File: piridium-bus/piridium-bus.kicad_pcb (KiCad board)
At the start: 2 copper layers, 90.2 x 95.9 mm, 53 parts, among them J1 EPS, J2 MODEM UART, J3 ANT, J4 PAYLOAD, Q1 2N7002, Q2 DMP3015LSSQ, U1 LM1117-3.3, U2 TPS54394RSAR, U3 MAX6369, U4 74LS126, U5 DS3232M

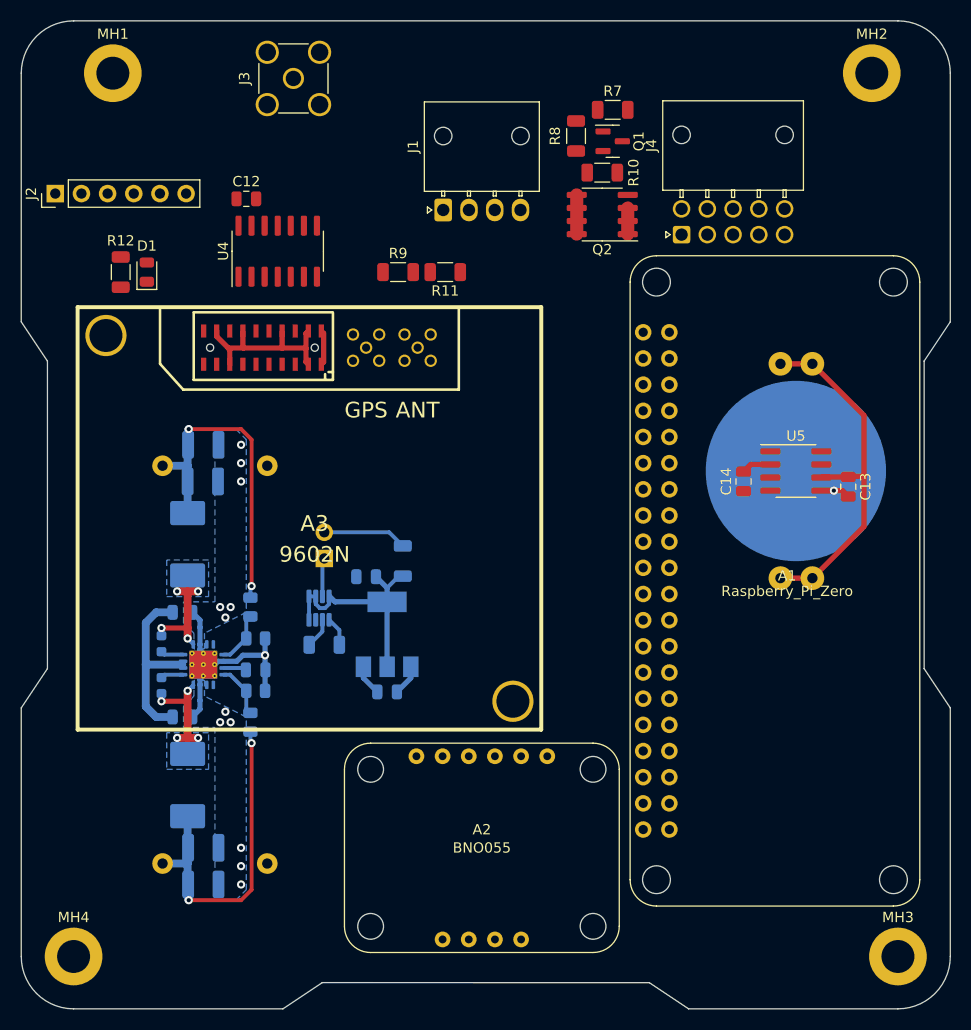
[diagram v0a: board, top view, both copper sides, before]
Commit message: update routing
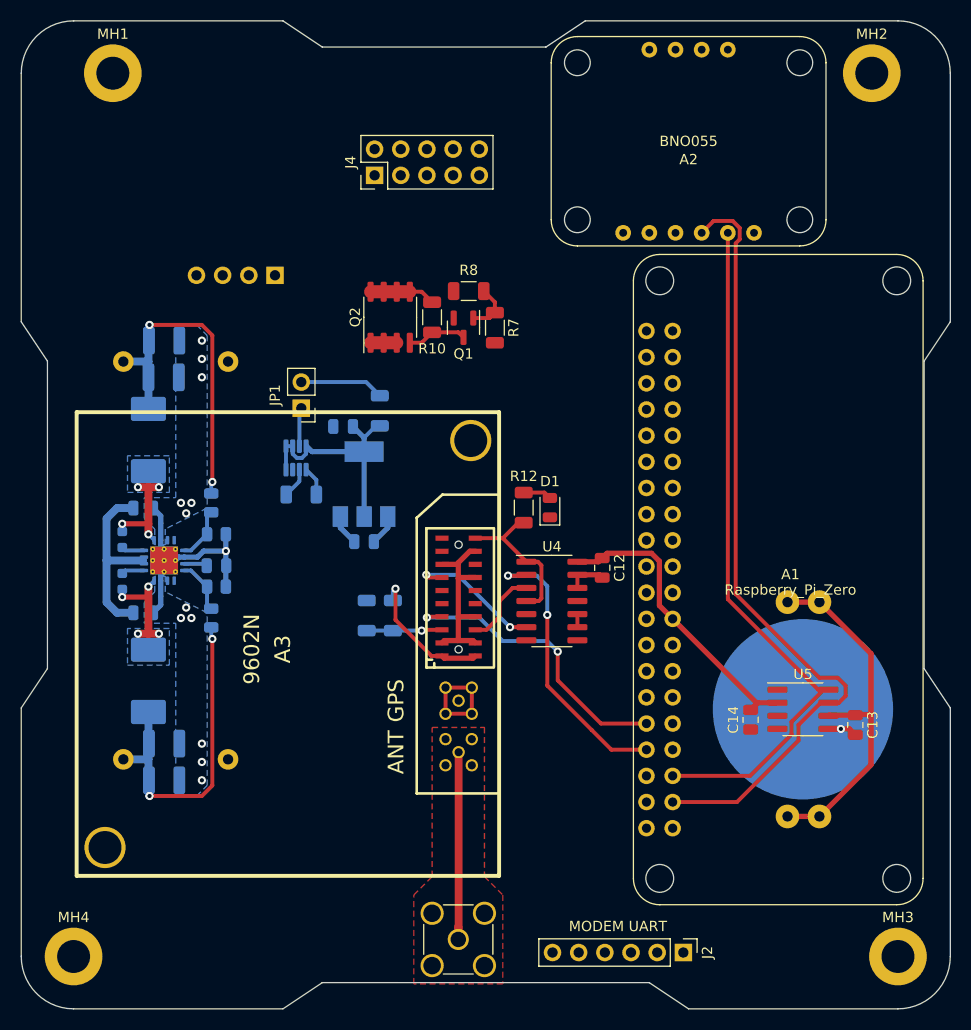
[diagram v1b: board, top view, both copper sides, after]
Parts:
- J1: footprint Connector_Molex:Molex_Nano-Fit_105313-xx04_1x04_P2.50mm_Horizontal -> Connector_PinHeader_2.54mm:PinHeader_1x04_P2.54mm_Horizontal; moved to B.Cu
- J4: footprint Connector_Molex:Molex_Nano-Fit_105314-xx10_2x05_P2.50mm_Horizontal -> Connector_PinHeader_2.54mm:PinHeader_2x05_P2.54mm_Vertical
- JP1: moved to F.Cu
- R11, R9: moved to B.Cu
- moved J2 95.6 mm to (165.9, 141.2), turned to -90 degrees
- moved J3 85.1 mm to (144.0, 140.0), turned to 180 degrees
- moved A2 71.5 mm to (166.4, 62.5), turned to 0 degrees
- moved C12 49.8 mm to (158.0, 103.9), turned to -90 degrees
- moved R12 45.3 mm to (150.4, 98.0)
- moved D1 45.3 mm to (152.9, 98.0)
- moved U4 43.1 mm to (153.1, 107.1), turned to 0 degrees
- moved A3 42.2 mm to (148.0, 88.8), turned to -90 degrees
- moved R11 34.2 mm to (135.1, 108.5), turned to -90 degrees
- moved R9 33.3 mm to (137.7, 108.5), turned to -90 degrees
- moved J4 30.3 mm to (135.9, 65.8)
- moved R7 24.0 mm to (147.6, 80.6), turned to -90 degrees
- moved Q1 23.2 mm to (144.5, 80.6), turned to -90 degrees
- moved BT1 23.1 mm to (177.5, 117.6)
- moved C13 23.1 mm to (182.6, 119.1)
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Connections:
- A3 pad 22: GND -> GNDS
- J3 pad 2: GND -> GNDS
- J4 pad 2: SPI_MOSI -> I2C_SCL
- J4 pad 3: SPI_MISO -> SPI_MOSI
- J4 pad 4: SPI_SCK -> I2C_SDA
- J4 pad 5: GND -> SPI_MISO
- J4 pad 6: I2C_SCL -> SPI_CE0
- J4 pad 7: I2C_SDA -> SPI_SCK
- J4 pad 8: SPI_CE0 -> SPI_CE1
- J4 pad 9: SPI_CE1 -> GND
- R9 pad 1: +5V -> +5VP
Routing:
- net I2C_SDA: track 0.00 -> 77.4 mm
- net I2C_SCL: track 0.00 -> 68.3 mm
- net UART_RX: track 0.00 -> 28.7 mm, vias 0 -> 2
- net UART_TX: track 0.00 -> 27.9 mm, vias 0 -> 2
- net +3.3V: track 2.90 -> 30.2 mm
- net Net-(A3-Pad21): track 0.00 -> 19.5 mm
- net /SUP_OUT: track 0.00 -> 14.9 mm
- net Net-(A3-Pad13): track 0.00 -> 13.5 mm, vias 0 -> 2
- net +5VP: track 35.9 -> 46.2 mm, vias 2 -> 3
- net unconnected-(A3-Pad24): track 0.00 -> 10.2 mm
- net Net-(A3-Pad6): track 0.00 -> 7.54 mm
- net S_MODEM_ON_OFF: track 0.00 -> 7.34 mm, vias 0 -> 1
- net Net-(Q1-Pad3): track 0.00 -> 5.83 mm
- net GND: track 46.1 -> 51.1 mm
- net Net-(Q1-Pad1): track 0.00 -> 4.86 mm
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- added copper zone on F.Cu, net GNDS
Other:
- outline, holes or cut-outs redrawn
